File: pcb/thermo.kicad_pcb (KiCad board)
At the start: 2 copper layers, 29 parts, among them J1 DB15_Female, J2 Barrel_Jack, U1 BME280

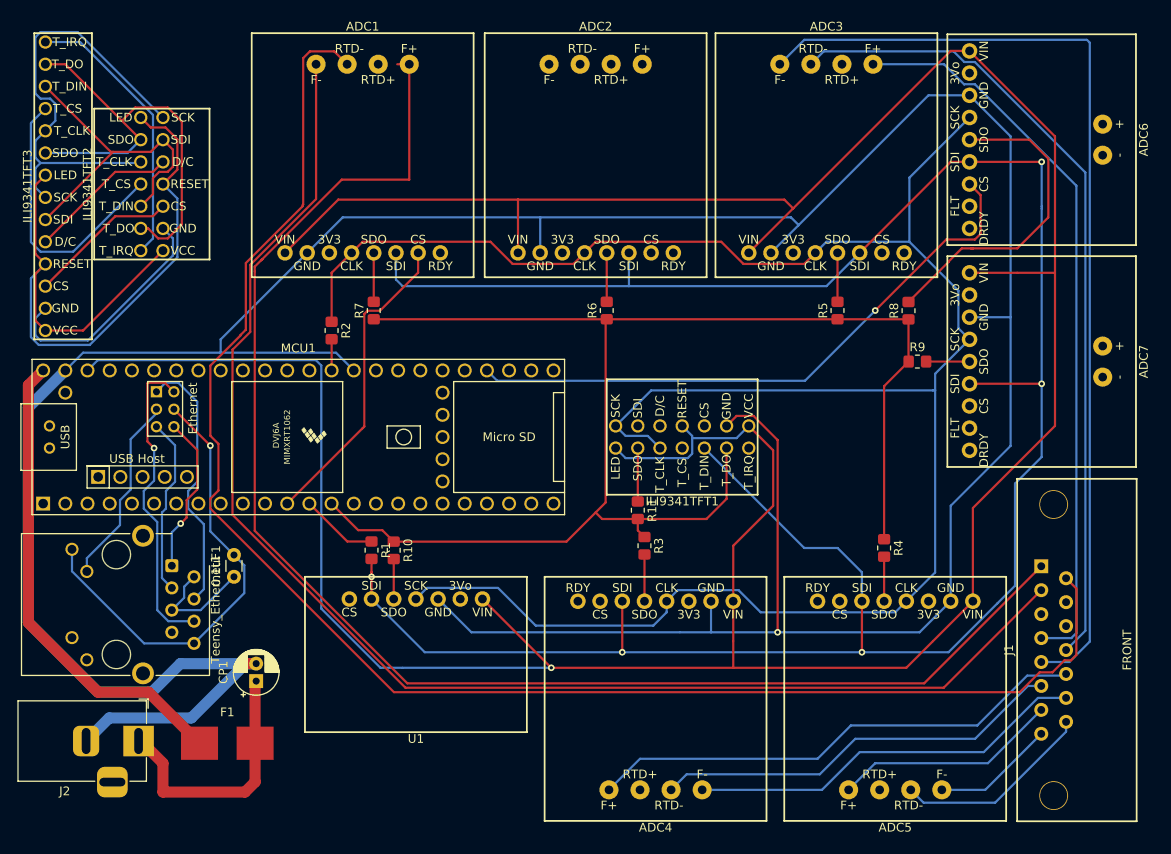
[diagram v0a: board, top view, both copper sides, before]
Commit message: Updated to latest specs
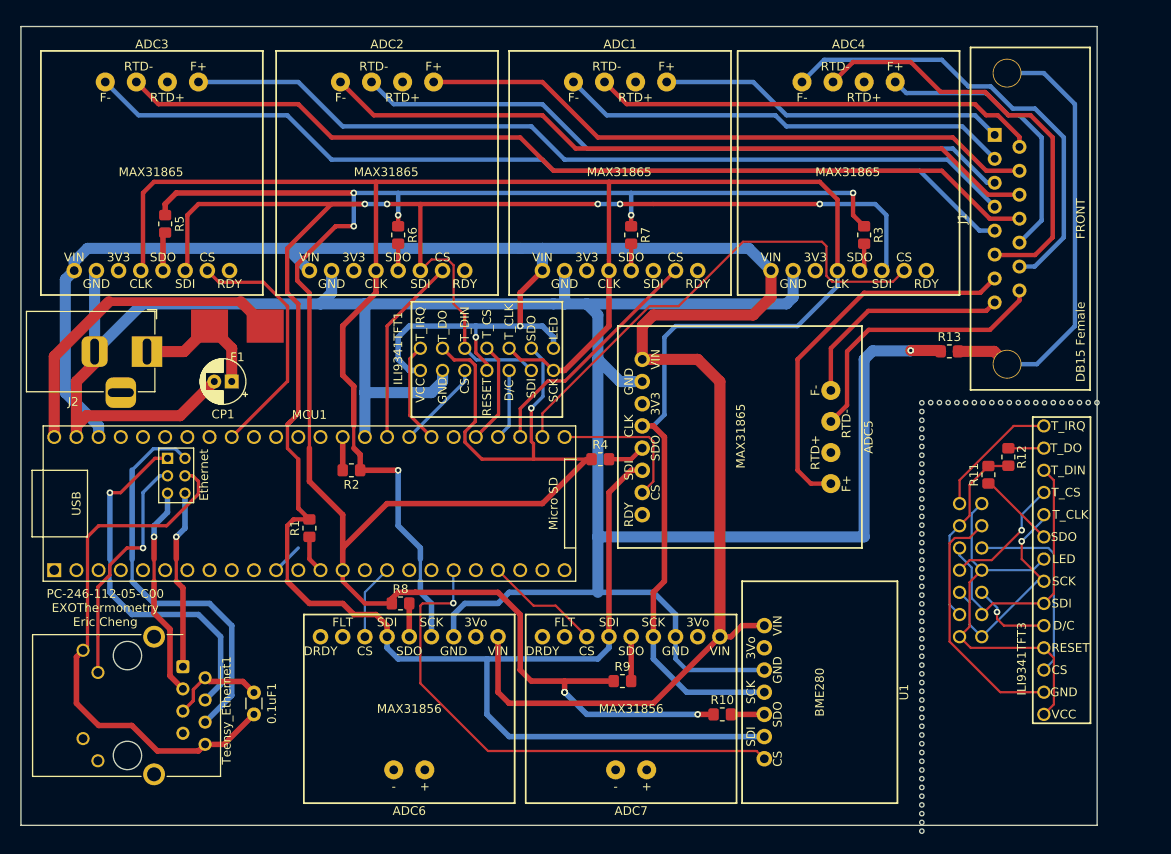
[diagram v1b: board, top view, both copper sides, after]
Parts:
- added R12: 22, Resistor_SMD:R_0805_2012Metric_Pad1.20x1.40mm_HandSolder, F.Cu at (130.8, 110.2)
- added R13: 0, Resistor_SMD:R_0805_2012Metric_Pad1.20x1.40mm_HandSolder, F.Cu at (124.1, 98.1)
- added REF**: VAL**, Thermometry:z_Drill_05x10, F.Cu at (120.9, 148.6)
- added REF**: VAL**, Thermometry:z_Drill_05x10, F.Cu at (120.9, 138.6)
- added REF**: VAL**, Thermometry:z_Drill_05x10, F.Cu at (120.9, 128.5)
- added REF**: VAL**, Thermometry:z_Drill_05x10, F.Cu at (120.9, 118.5)
- added REF**: VAL**, Thermometry:z_Drill_05x10, F.Cu at (120.9, 108.5)
- added REF**: VAL**, Thermometry:z_Drill_05x10, F.Cu at (126.4, 104.0)
- added REF**: VAL**, Thermometry:z_Drill_05x10, F.Cu at (136.4, 104.0)
- ILI9341TFT2: moved to B.Cu
- moved ILI9341TFT3 122.5 mm to (134.9, 123.2)
- moved ILI9341TFT2 103.6 mm to (126.5, 123.2), turned to 270 degrees
- moved ADC6 97.4 mm to (62.2, 139.1), turned to 180 degrees
- moved R5 77.6 mm to (34.3, 83.5), turned to 270 degrees
- moved ADC3 77.2 mm to (32.8, 77.7)
- moved R8 67.1 mm to (61.2, 127.0), turned to 0 degrees
- moved ADC4 64.1 mm to (112.5, 77.7), turned to 0 degrees
- moved ADC7 61.5 mm to (87.6, 139.1), turned to 180 degrees
- moved R9 49.8 mm to (86.6, 135.9)
- moved J1 49.7 mm to (132.1, 83.0)
- moved F1 47.8 mm to (42.6, 95.2), turned to 180 degrees
- moved U1 46.4 mm to (109.2, 137.2), turned to 270 degrees
- moved J2 44.6 mm to (32.2, 98.2)
- moved R3 43.6 mm to (114.3, 84.8)
- moved R10 42.0 mm to (98.1, 139.7), turned to 0 degrees
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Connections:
- ILI9341TFT1 pad 9: Net-(ILI9341TFT1-Pad9) -> /SDO
- ILI9341TFT3 pad 13: /SDO -> Net-(ILI9341TFT3-Pad13)
- ILI9341TFT3 pad 9: /SDO -> Net-(ILI9341TFT3-Pad9)
- J1 pad 0: (no net) -> Net-(J1-Pad0)
- MCU1 pad 10: /CS_5 -> Net-(MCU1-Pad10)
- MCU1 pad 11: /TFT_DC -> Net-(MCU1-Pad11)
- MCU1 pad 12: /CS_1 -> Net-(MCU1-Pad12)
- MCU1 pad 16: Net-(MCU1-Pad16) -> /CS_6
- MCU1 pad 19: Net-(MCU1-Pad19) -> /CS_8
- MCU1 pad 21: Net-(MCU1-Pad21) -> /CS_7
- MCU1 pad 25: /T_IRQ -> /CS_5
- MCU1 pad 26: /T_CS -> /CS_4
- MCU1 pad 27: /TFT_CS -> /CS_1
- MCU1 pad 28: /CS_6 -> /TFT_DC
- MCU1 pad 29: /CS_7 -> /T_CS
- MCU1 pad 30: /CS_8 -> Net-(MCU1-Pad30)
- MCU1 pad 31: Net-(MCU1-Pad31) -> /T_IRQ
- MCU1 pad 32: Net-(MCU1-Pad32) -> /TFT_CS
- MCU1 pad 33: Net-(MCU1-Pad33) -> /CS_2
- MCU1 pad 40: Net-(MCU1-Pad40) -> /CS_3
- MCU1 pad 7: /CS_2 -> Net-(MCU1-Pad7)
- MCU1 pad 8: /CS_3 -> Net-(MCU1-Pad8)
- MCU1 pad 9: /CS_4 -> Net-(MCU1-Pad9)
- R11 pad 1: Net-(ILI9341TFT1-Pad9) -> Net-(ILI9341TFT3-Pad9)
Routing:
- net +3V3: track 468.3 -> 295.1 mm, vias 1 -> 2
- net Net-(ADC1-Pad10): track 181.6 -> 51.2 mm
- net Net-(ADC1-Pad12): track 169.6 -> 40.1 mm
- net Net-(ADC1-Pad9): track 160.9 -> 51.9 mm
- net GND: track 417.7 -> 332.1 mm
- net Net-(ADC2-Pad9): track 0.00 -> 83.2 mm
- net /SDO: track 220.3 -> 300.6 mm, vias 0 -> 9
- net Net-(ADC2-Pad10): track 0.00 -> 76.1 mm
- net Net-(ADC2-Pad12): track 0.00 -> 71.3 mm
- net /CS_6: track 70.2 -> 8.67 mm, vias 1 -> 0
- net /CS_8: track 0.00 -> 59.6 mm, vias 0 -> 1
- net /CS_4: track 0.00 -> 56.7 mm
- net Net-(J1-Pad0): track 0.00 -> 50.4 mm
- net Net-(ADC6-Pad5): track 36.9 -> 3.81 mm
- net /CS_3: track 0.00 -> 28.5 mm
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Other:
- board outline added: 123.2 x 91.4 mm
- board text added: "PC-246-112-05-C00 EXOThermometry Eric Cheng"
